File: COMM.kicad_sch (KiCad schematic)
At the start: 4 parts

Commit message: OBC: preliminary layout
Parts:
- MH5, MH6, MH7, MH8: footprint MountingHole-VST104:MountingHole_3.2mm_M3_Pad_Via -> MountingHole:MountingHole_3.2mm_M3_Pad_Via
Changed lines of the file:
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@@
 			)
 		)
-		(property "Footprint" "MountingHole-VST104:MountingHole_3.2mm_M3_Pad_Via"
+		(property "Footprint" "MountingHole:MountingHole_3.2mm_M3_Pad_Via"
 			(at 312.42 223.52 0)
 			(effects
@@
 			)
 		)
-		(property "Footprint" "MountingHole-VST104:MountingHole_3.2mm_M3_Pad_Via"
+		(property "Footprint" "MountingHole:MountingHole_3.2mm_M3_Pad_Via"
 			(at 308.61 217.17 0)
 			(effects
@@
 			)
 		)
-		(property "Footprint" "MountingHole-VST104:MountingHole_3.2mm_M3_Pad_Via"
+		(property "Footprint" "MountingHole:MountingHole_3.2mm_M3_Pad_Via"
 			(at 326.39 223.52 0)
 			(effects
@@
 		(dnp no)
 		(fields_autoplaced yes)
-		(property "Reference" "#PWR068"
+		(property "Reference" "#PWR039"
 			(at 320.04 234.95 0)
 			(effects
@@
 			(project "Avionics"
 				(path "/ace5002f-3cbc-4a0a-869b-0e31ebd905b7/617751c8-9e63-43a2-807c-be0203e52cd6"
-					(reference "#PWR068")
+					(reference "#PWR039")
 					(unit 1)
 				)
@@
 			)
 		)
-		(property "Footprint" "MountingHole-VST104:MountingHole_3.2mm_M3_Pad_Via"
+		(property "Footprint" "MountingHole:MountingHole_3.2mm_M3_Pad_Via"
 			(at 321.31 217.17 0)
 			(effects

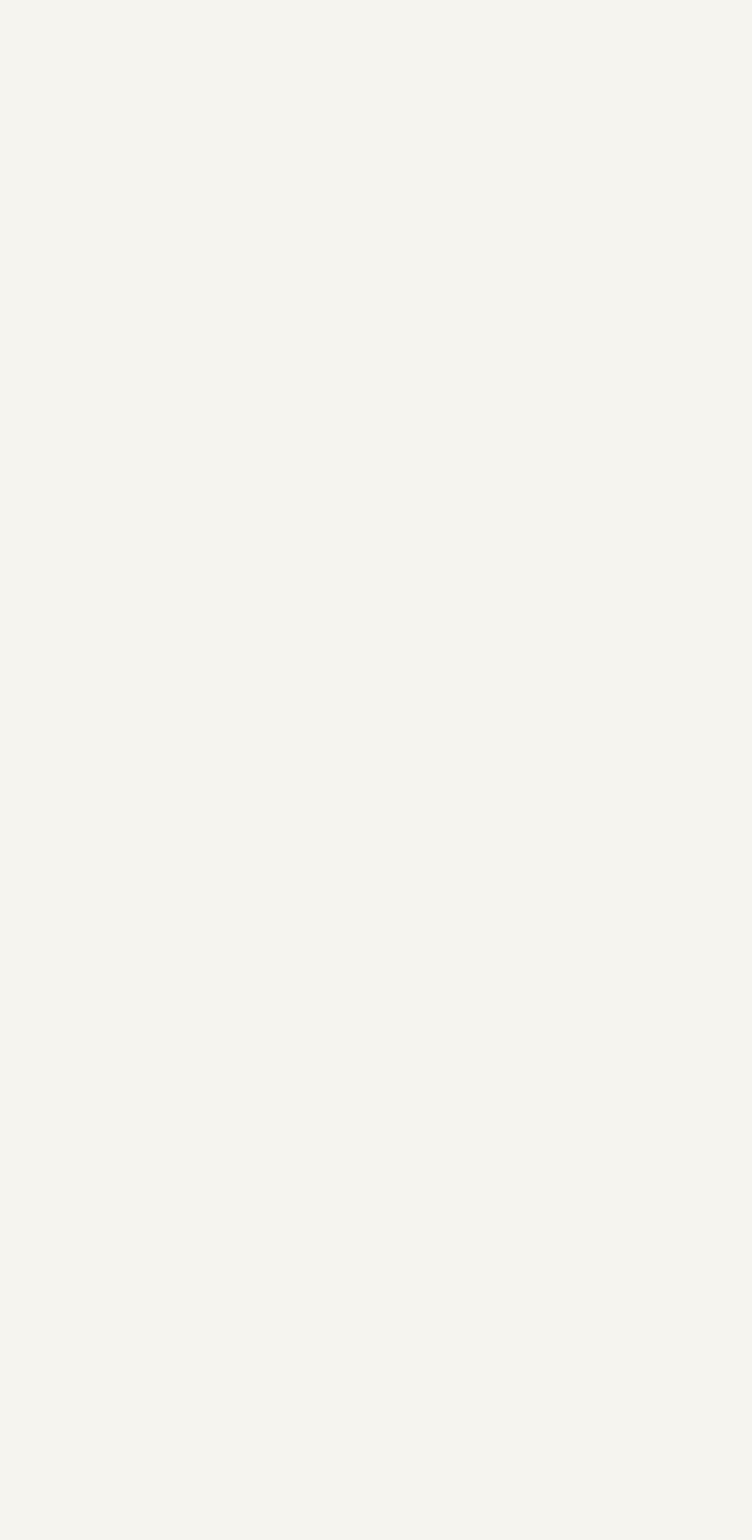
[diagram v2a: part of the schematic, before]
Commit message: OBC: Continue PCB lauout
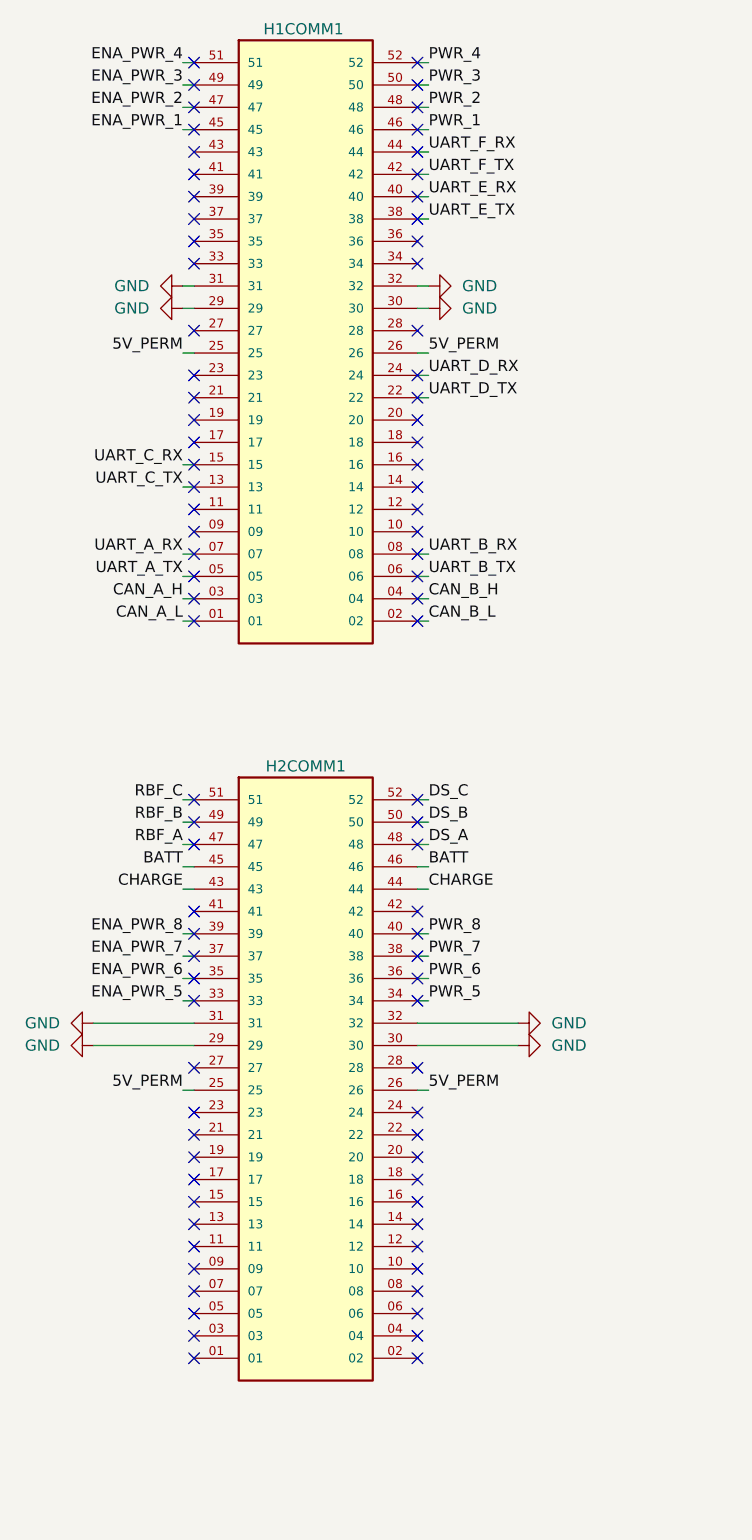
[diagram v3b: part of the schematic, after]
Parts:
- added H1COMM1, H2COMM1: Conn_02x26_Odd_Even, ESQ-126-39-G-D:SAMTEC_ESQ-126-39-G-D, symbol ESQ-126-39-G-D:ESQ-126-39-G-D
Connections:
- net GND: now also H1COMM1.29, H1COMM1.30, H1COMM1.31, H1COMM1.32, H2COMM1.29, H2COMM1.30, H2COMM1.31, H2COMM1.32
- new net 5V_PERM: H1COMM1.25, H1COMM1.26, H2COMM1.25, H2COMM1.26
- new net BATT: H2COMM1.45, H2COMM1.46
- new net CAN_A_H: H1COMM1.03
- new net CAN_A_L: H1COMM1.01
- new net CAN_B_H: H1COMM1.04
- new net CAN_B_L: H1COMM1.02
- new net CHARGE: H2COMM1.43, H2COMM1.44
- new net DS_A: H2COMM1.48
- new net DS_B: H2COMM1.50
- new net DS_C: H2COMM1.52
- new net ENA_PWR_1: H1COMM1.45
- new net ENA_PWR_2: H1COMM1.47
- new net ENA_PWR_3: H1COMM1.49
- new net ENA_PWR_4: H1COMM1.51
- new net ENA_PWR_5: H2COMM1.33
- new net ENA_PWR_6: H2COMM1.35
- new net ENA_PWR_7: H2COMM1.37
- new net ENA_PWR_8: H2COMM1.39
- new net PWR_1: H1COMM1.46
- new net PWR_2: H1COMM1.48
- new net PWR_3: H1COMM1.50
- new net PWR_4: H1COMM1.52
- new net PWR_5: H2COMM1.34
- new net PWR_6: H2COMM1.36
- new net PWR_7: H2COMM1.38
- new net PWR_8: H2COMM1.40
- new net RBF_A: H2COMM1.47
- new net RBF_B: H2COMM1.49
- new net RBF_C: H2COMM1.51
- new net UART_A_RX: H1COMM1.07
- new net UART_A_TX: H1COMM1.05
- new net UART_B_RX: H1COMM1.08
- new net UART_B_TX: H1COMM1.06
- new net UART_C_RX: H1COMM1.15
- new net UART_C_TX: H1COMM1.13
- new net UART_D_RX: H1COMM1.24
- new net UART_D_TX: H1COMM1.22
- new net UART_E_RX: H1COMM1.40
- new net UART_E_TX: H1COMM1.38
- new net UART_F_RX: H1COMM1.44
- new net UART_F_TX: H1COMM1.42
- no-connect marks 0 -> 88
